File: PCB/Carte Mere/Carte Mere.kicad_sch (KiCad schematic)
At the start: 0 parts

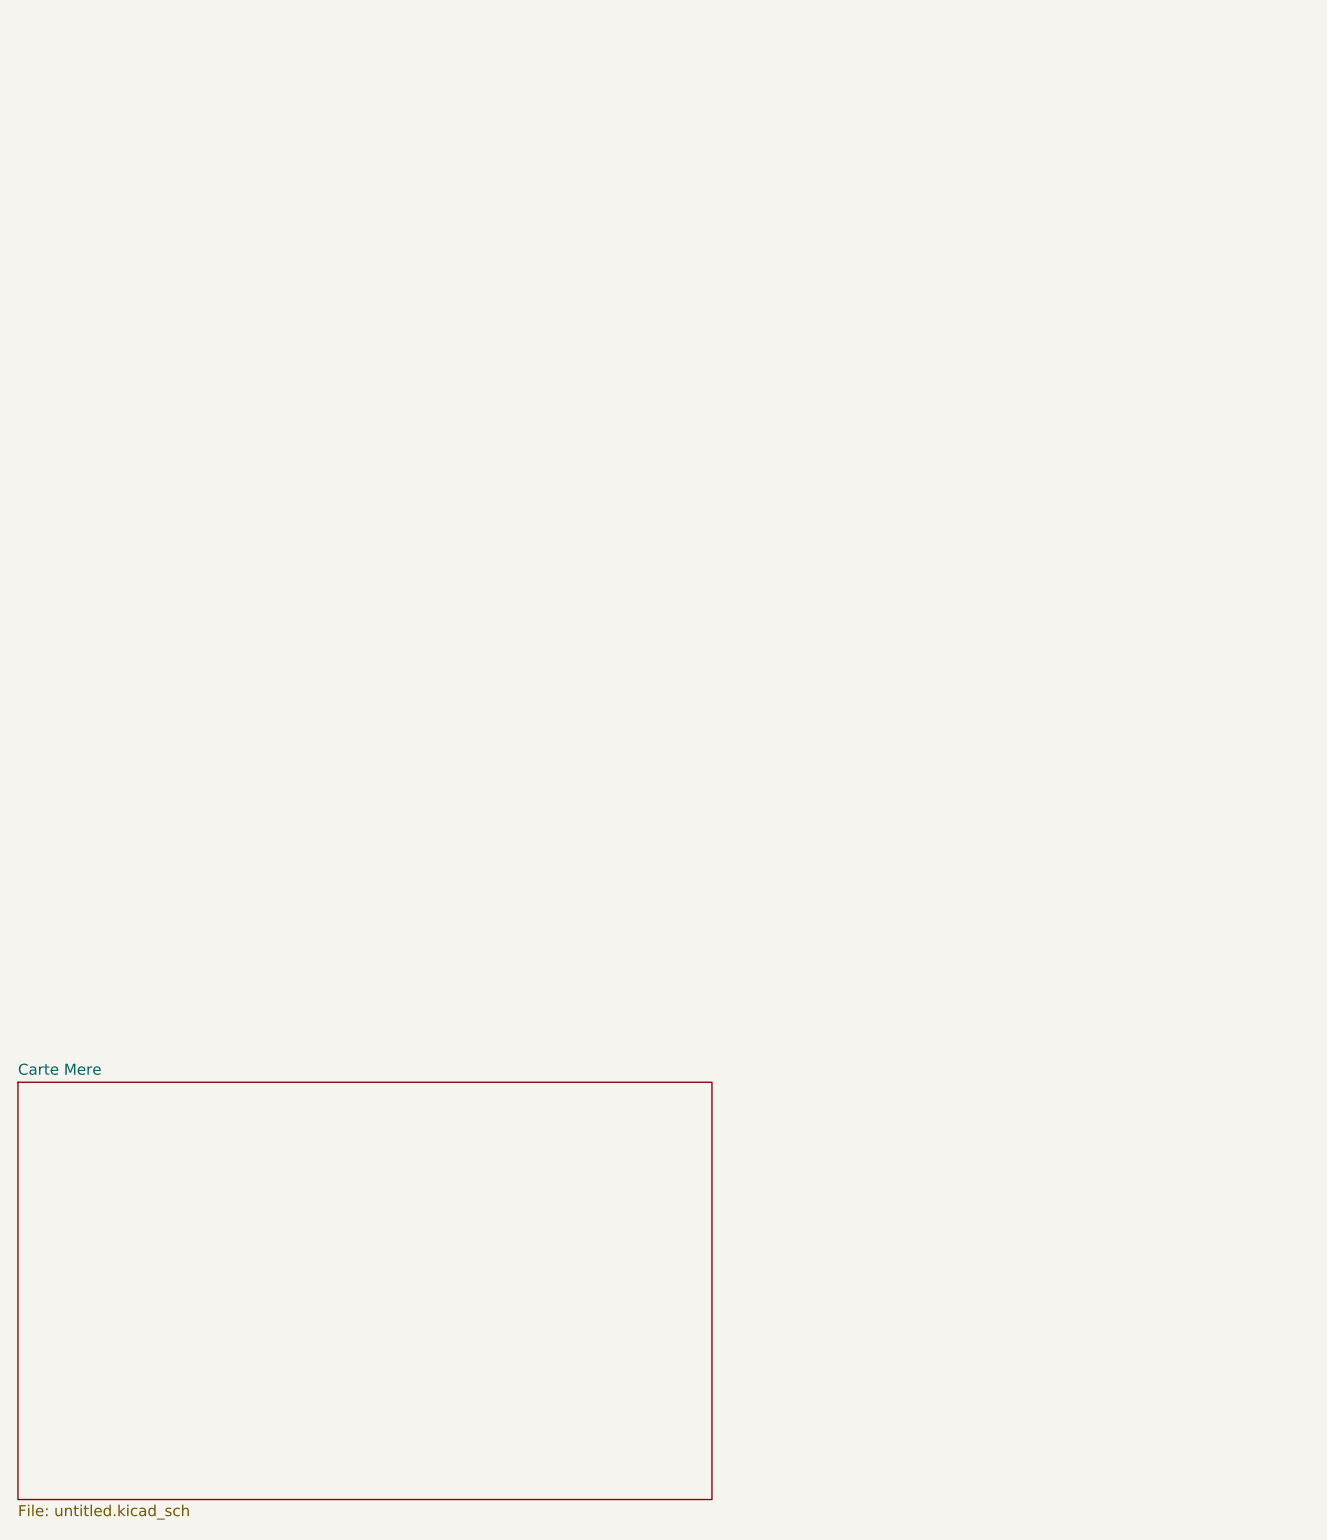
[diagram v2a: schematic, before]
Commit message: 1.2 PCB
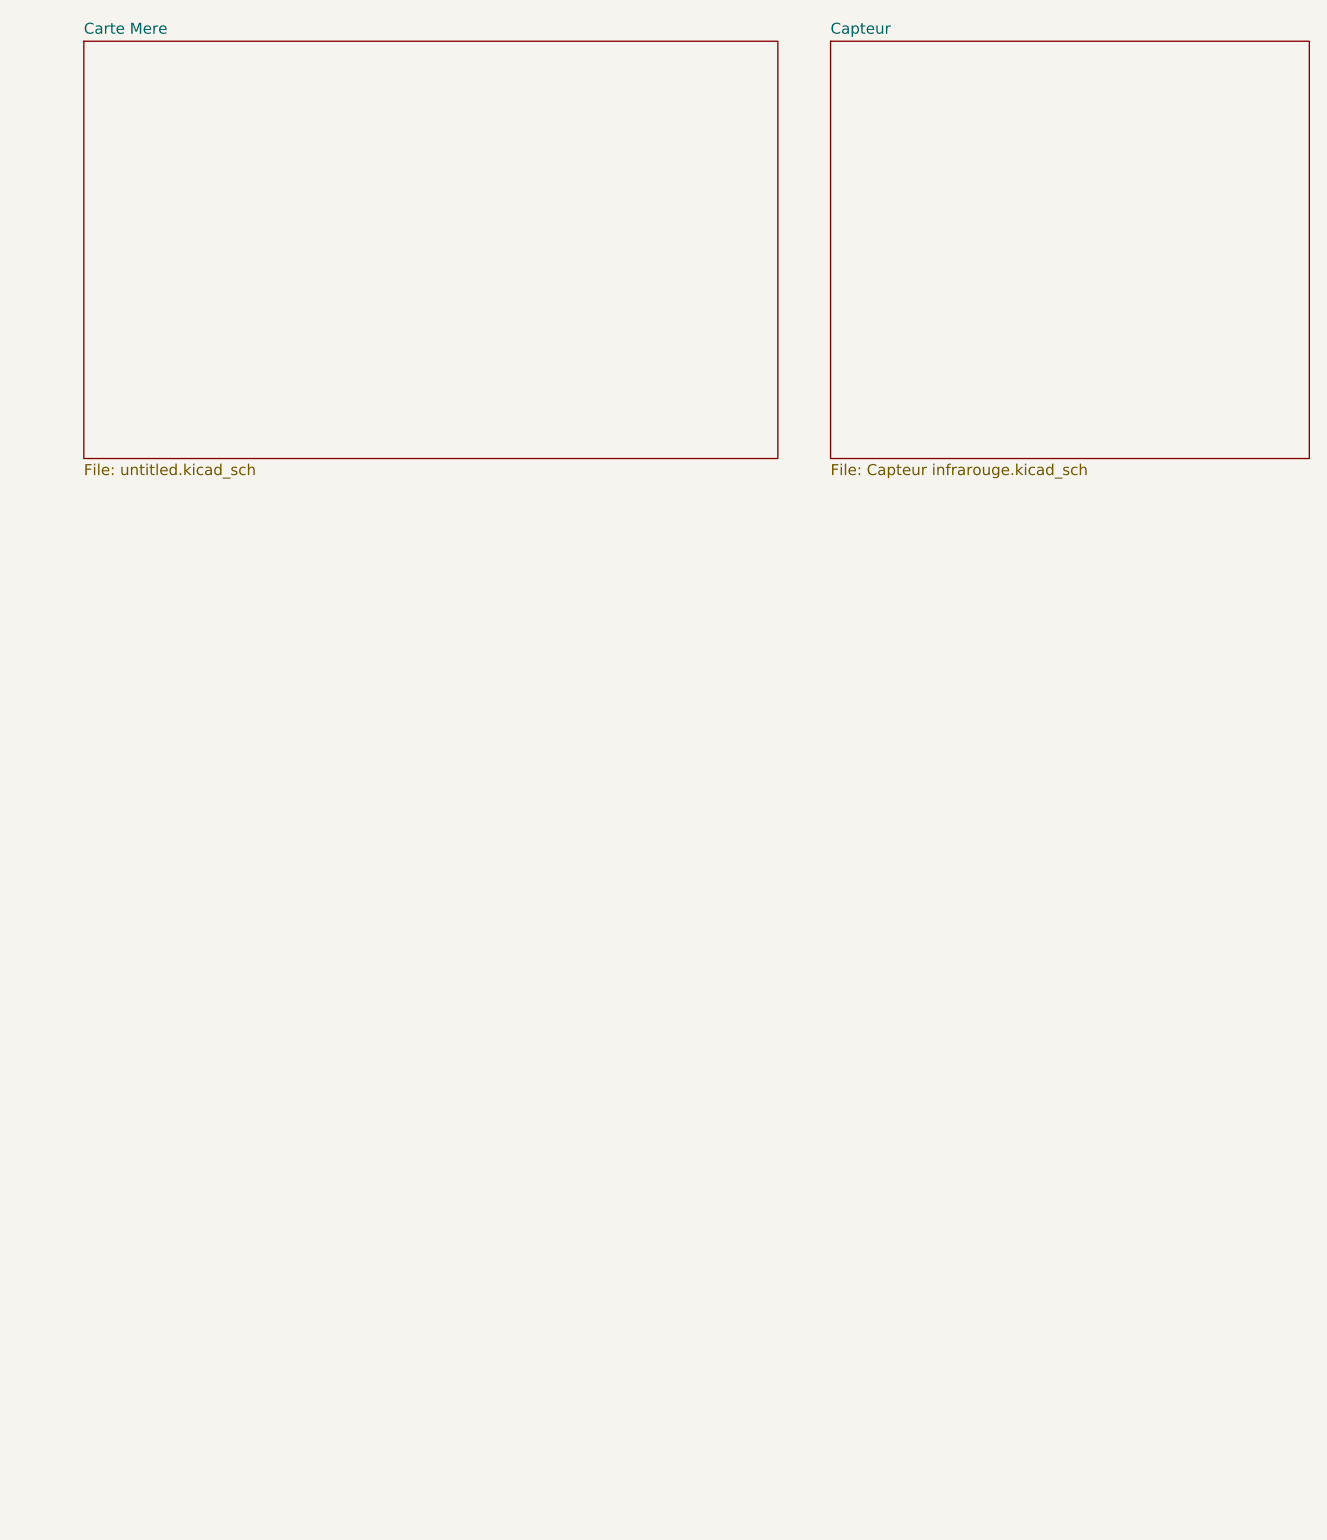
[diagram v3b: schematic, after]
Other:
- added sheet Capteur (Capteur infrarouge.kicad_sch)
